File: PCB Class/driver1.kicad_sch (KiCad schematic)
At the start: 16 parts, among them U3 MAX7219, U4 MAX7219, U5 MAX7219, U6 MAX7219

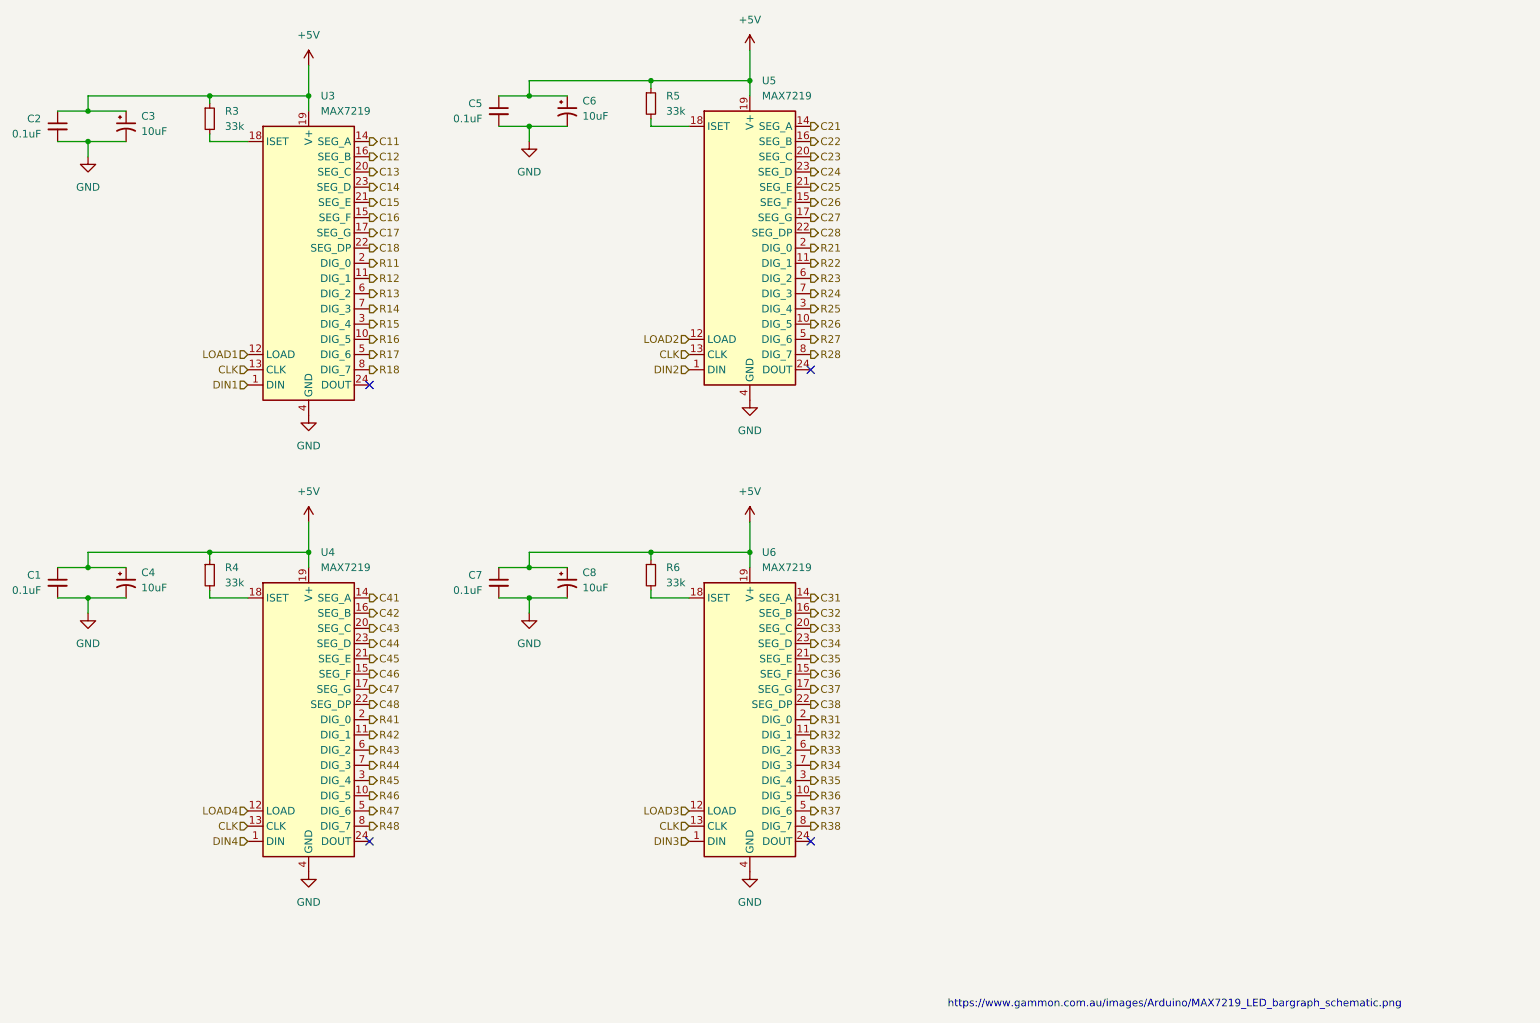
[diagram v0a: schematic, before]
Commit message: Footprints
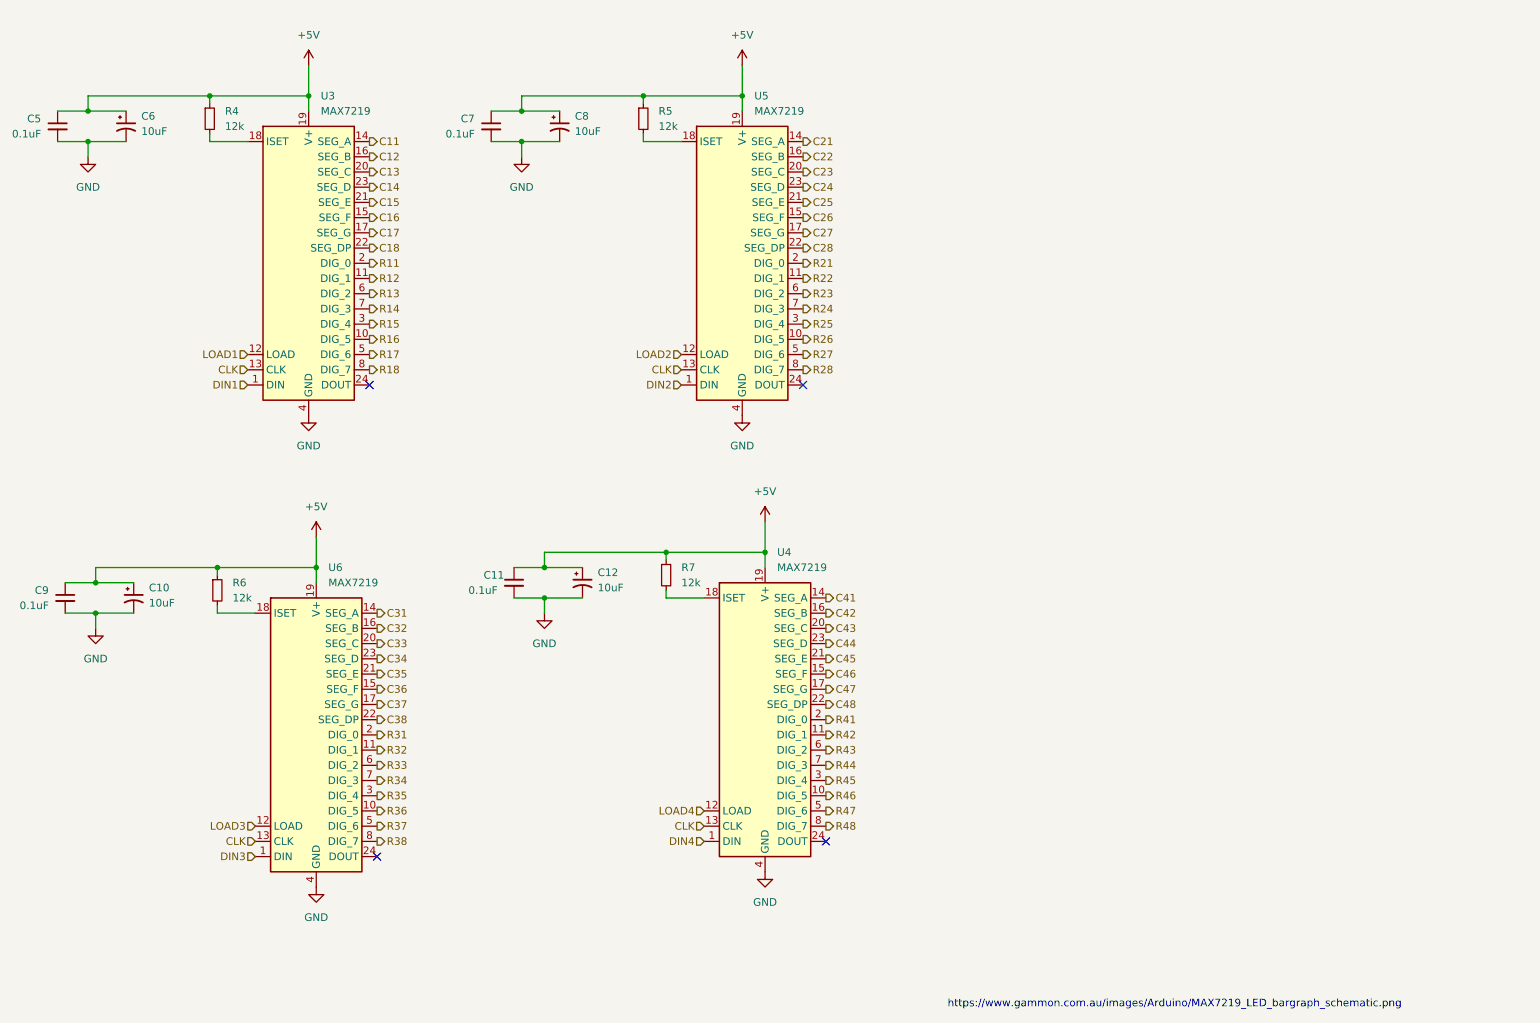
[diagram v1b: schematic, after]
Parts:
- C10: renamed from C8; footprint (none) -> Capacitor_SMD:C_0603_1608Metric
- C11: renamed from C1; footprint (none) -> Capacitor_SMD:C_0603_1608Metric
- C12: renamed from C4; footprint (none) -> Capacitor_SMD:C_0603_1608Metric
- C5: renamed from C2; footprint (none) -> Capacitor_SMD:C_0603_1608Metric
- C6: renamed from C3; footprint (none) -> Capacitor_SMD:C_0603_1608Metric
- C7: renamed from C5; footprint (none) -> Capacitor_SMD:C_0603_1608Metric
- C8: renamed from C6; footprint (none) -> Capacitor_SMD:C_0603_1608Metric
- C9: renamed from C7; footprint (none) -> Capacitor_SMD:C_0603_1608Metric
- R4: renamed from R3; value 33k -> 12k; footprint (none) -> Resistor_SMD:R_0603_1608Metric
- R5, R6: value 33k -> 12k; footprint (none) -> Resistor_SMD:R_0603_1608Metric
- R7: renamed from R4; value 33k -> 12k; footprint (none) -> Resistor_SMD:R_0603_1608Metric
- U3, U4, U5, U6: footprint (none) -> MAX7219:SOIC24
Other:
- moved on the sheet: C10, C11, C12, C7, C8, C9, R5, R6, R7, U4, U5, U6
